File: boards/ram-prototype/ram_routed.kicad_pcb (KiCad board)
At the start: 4 copper layers, 217 x 107 mm, 512 parts, among them J1 PinHeader_1x16_P2\.54mm_Verti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, U1 DSBGA\-5_NumericPads, U10 DSBGA\-6_NumericPads, U100 DSBGA\-5_NumericPads, U101 DSBGA\-5_NumericPads, U102 DSBGA\-5_NumericPads, U103 DSBGA\-5_NumericPads, U104 DSBGA\-5_NumericPads, U105 DSBGA\-5_NumericPads, U106 DSBGA\-5_NumericPads, U107 DSBGA\-5_NumericPads, U108 DSBGA\-5_NumericPads, U109 DSBGA\-5_NumericPads, U11 DSBGA\-6_NumericPads, U110 DSBGA\-5_NumericPads, U111 DSBGA\-5_NumericPads, U112 DSBGA\-5_NumericPads, U113 DSBGA\-5_NumericPads, U114 DSBGA\-5_NumericPads, U115 DSBGA\-5_NumericPads, U116 DSBGA\-5_NumericPads, U117 DSBGA\-5_NumericPads, U118 DSBGA\-5_NumericPads, U119 DSBGA\-5_NumericPads, U12 DSBGA\-5_NumericPads, U120 DSBGA\-5_NumericPads, U121 DSBGA\-5_NumericPads, U122 DSBGA\-5_NumericPads, U123 DSBGA\-5_NumericPads, U124 DSBGA\-5_NumericPads, U125 DSBGA\-5_NumericPads, U126 DSBGA\-5_NumericPads, U127 DSBGA\-5_NumericPads, U128 DSBGA\-5_NumericPads, U129 DSBGA\-5_NumericPads, U13 DSBGA\-5_NumericPads, U130 DSBGA\-5_NumericPads, U131 DSBGA\-5_NumericPads, U132 DSBGA\-5_NumericPads, U133 DSBGA\-5_NumericPads, U134 DSBGA\-5_NumericPads, U135 DSBGA\-5_NumericPads, U136 DSBGA\-5_NumericPads, U137 DSBGA\-5_NumericPads, U138 DSBGA\-5_NumericPads, U139 DSBGA\-5_NumericPads, U14 DSBGA\-5_NumericPads, U140 DSBGA\-5_NumericPads, U141 DSBGA\-5_NumericPads, U142 DSBGA\-5_NumericPads, U143 DSBGA\-5_NumericPads, U144 DSBGA\-5_NumericPads, U145 DSBGA\-5_NumericPads, U146 DSBGA\-5_NumericPads, U147 DSBGA\-5_NumericPads, U148 DSBGA\-5_NumericPads, U149 DSBGA\-5_NumericPads, U15 DSBGA\-5_NumericPads, U150 DSBGA\-5_NumericPads, U151 DSBGA\-5_NumericPads, U152 DSBGA\-5_NumericPads, U153 DSBGA\-5_NumericPads, U154 DSBGA\-5_NumericPads, U155 DSBGA\-5_NumericPads, U156 DSBGA\-5_NumericPads, U157 DSBGA\-5_NumericPads, U158 DSBGA\-5_NumericPads, U159 DSBGA\-5_NumericPads, U16 DSBGA\-5_NumericPads, U160 DSBGA\-5_NumericPads, U161 DSBGA\-5_NumericPads, U17 DSBGA\-5_NumericPads, U18 DSBGA\-5_NumericPads, U19 DSBGA\-5_NumericPads, U2 DSBGA\-5_NumericPads, U20 DSBGA\-5_NumericPads, U21 DSBGA\-5_NumericPads, U22 DSBGA\-5_NumericPads, U23 DSBGA\-5_NumericPads, U24 DSBGA\-5_NumericPads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

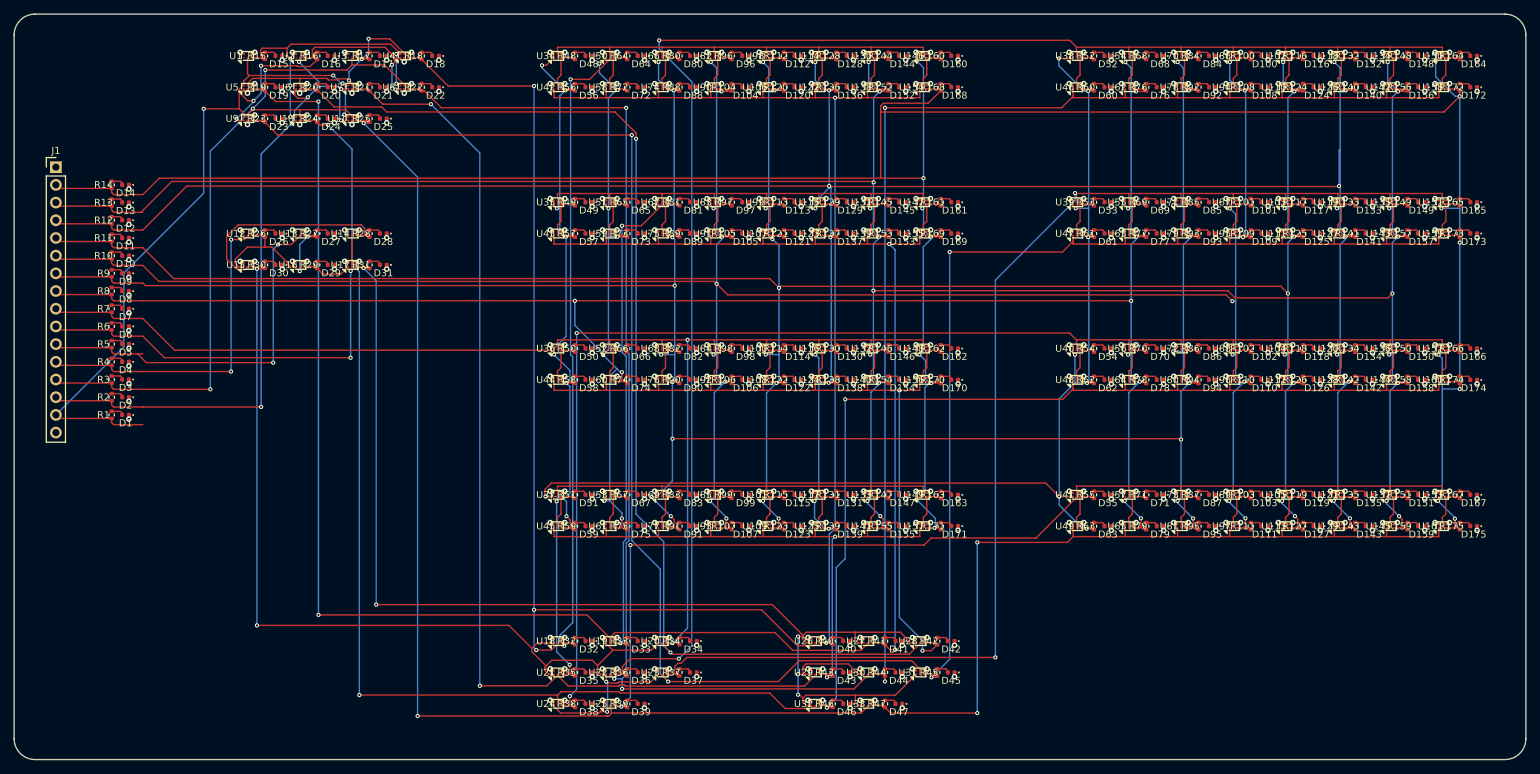
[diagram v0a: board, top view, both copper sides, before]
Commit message: rearange some components
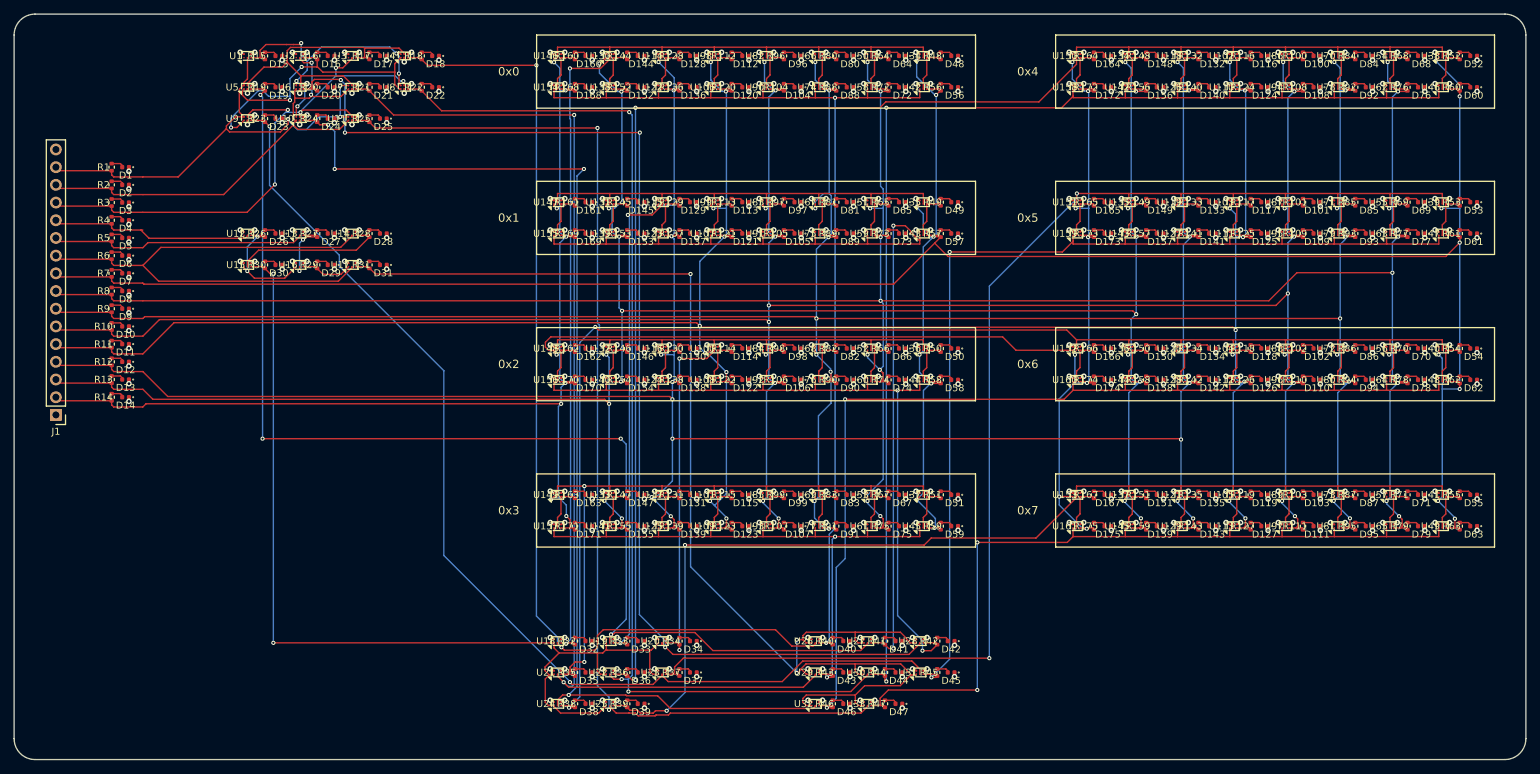
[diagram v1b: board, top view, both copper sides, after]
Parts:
- moved D160 52.5 mm to (95.5, 19.0)
- moved D161 52.5 mm to (95.5, 40.0)
- moved D162 52.5 mm to (95.5, 61.0)
- moved D163 52.5 mm to (95.5, 82.0)
- moved D164 52.5 mm to (170.0, 19.0)
- moved D165 52.5 mm to (170.0, 40.0)
- moved D166 52.5 mm to (170.0, 61.0)
- moved D167 52.5 mm to (170.0, 82.0)
- moved D168 52.5 mm to (95.5, 23.5)
- moved D169 52.5 mm to (95.5, 44.5)
- moved D170 52.5 mm to (95.5, 65.5)
- moved D171 52.5 mm to (95.5, 86.5)
- moved D172 52.5 mm to (170.0, 23.5)
- moved D173 52.5 mm to (170.0, 44.5)
- moved D174 52.5 mm to (170.0, 65.5)
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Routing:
- net /D7: track 410.5 -> 335.8 mm, vias 16 -> 17
- net /D0: track 340.4 -> 393.8 mm
- net /D6: track 369.6 -> 333.8 mm
- net /Address Decoder/A0: track 101.3 -> 67.3 mm, vias 4 -> 3
- net /D1: track 340.8 -> 373.0 mm
- net /D5: track 373.8 -> 342.4 mm, vias 18 -> 19
- net /Address Decoder/A1: track 99.4 -> 69.1 mm, vias 6 -> 2
- net /Address Decoder/A2: track 112.2 -> 84.9 mm, vias 3 -> 5
- net /Address Decoder/SEL5: track 176.2 -> 154.6 mm
- net /D2: track 342.5 -> 363.0 mm, vias 19 -> 18
- net /Control Logic/nCE: track 47.9 -> 29.6 mm, vias 2 -> 0
- net /Control Logic/nOE: track 54.5 -> 36.9 mm, vias 2 -> 0
- net /Control Logic/nWE: track 62.3 -> 77.3 mm, vias 2 -> 0
- net /Byte 4/WRITE_CLK: track 228.1 -> 217.1 mm
- net Net-(R28-Pad1): track 31.0 -> 21.9 mm
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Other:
- board text added: "0x0"
- board text added: "0x1"
- board text added: "0x2"
- board text added: "0x3"
- board text added: "0x4"
- board text added: "0x5"
- board text added: "0x6"
- board text added: "0x7"
